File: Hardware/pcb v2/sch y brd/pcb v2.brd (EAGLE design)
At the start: 80 x 80 mm, 60 parts, among them J1 AVR_SPI_PRG_6PTH, J2 1981584-1, J3 HDMI, J4 HDMI, J5 JST-3, Q1 PMBT3904, Q2 PMBT3904, Q4 MC-306, U1 ATMEGA328P, U2 TXS0108EPWR-TSSOP20, U3 MB85RS16N, U4 ADP3338AKCZ-3.3RL7, U5 DS1307SO8, Y2 CSTCE16M0V53-R0 16MHZ

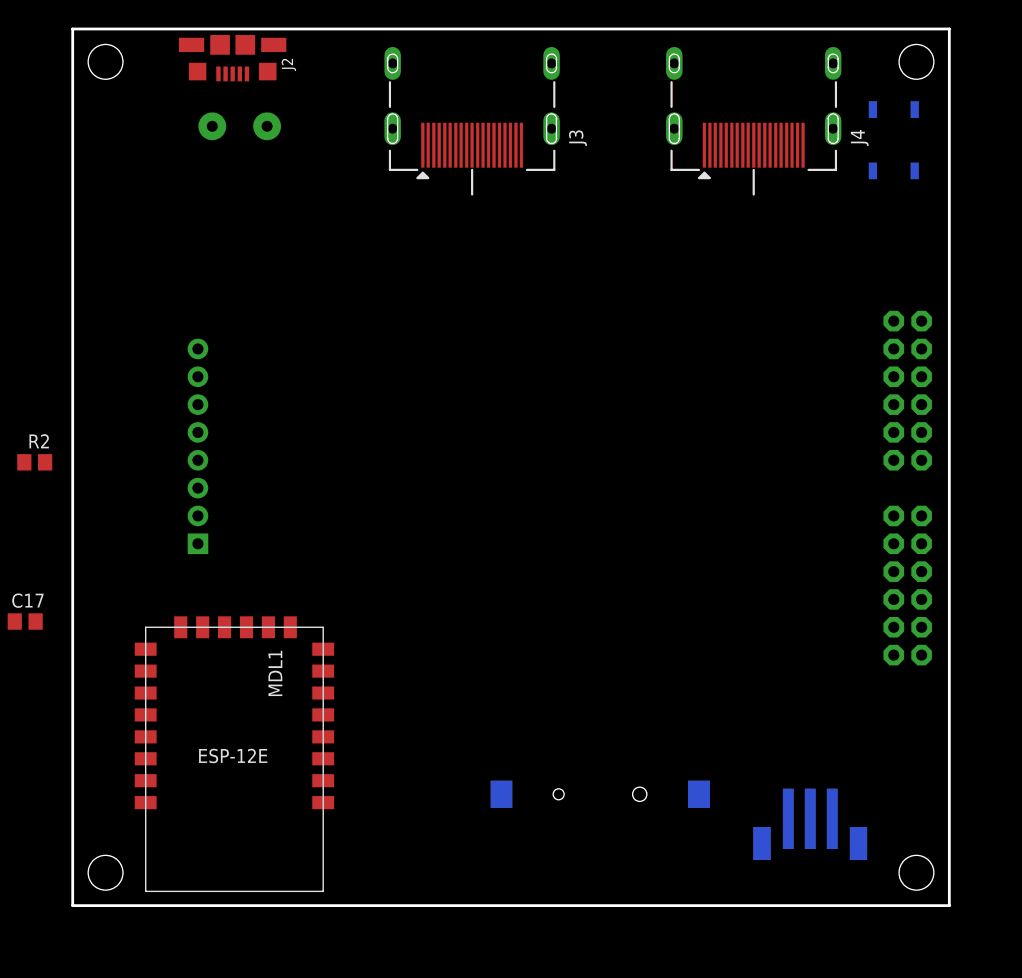
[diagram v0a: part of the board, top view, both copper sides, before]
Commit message: ruteo tdms
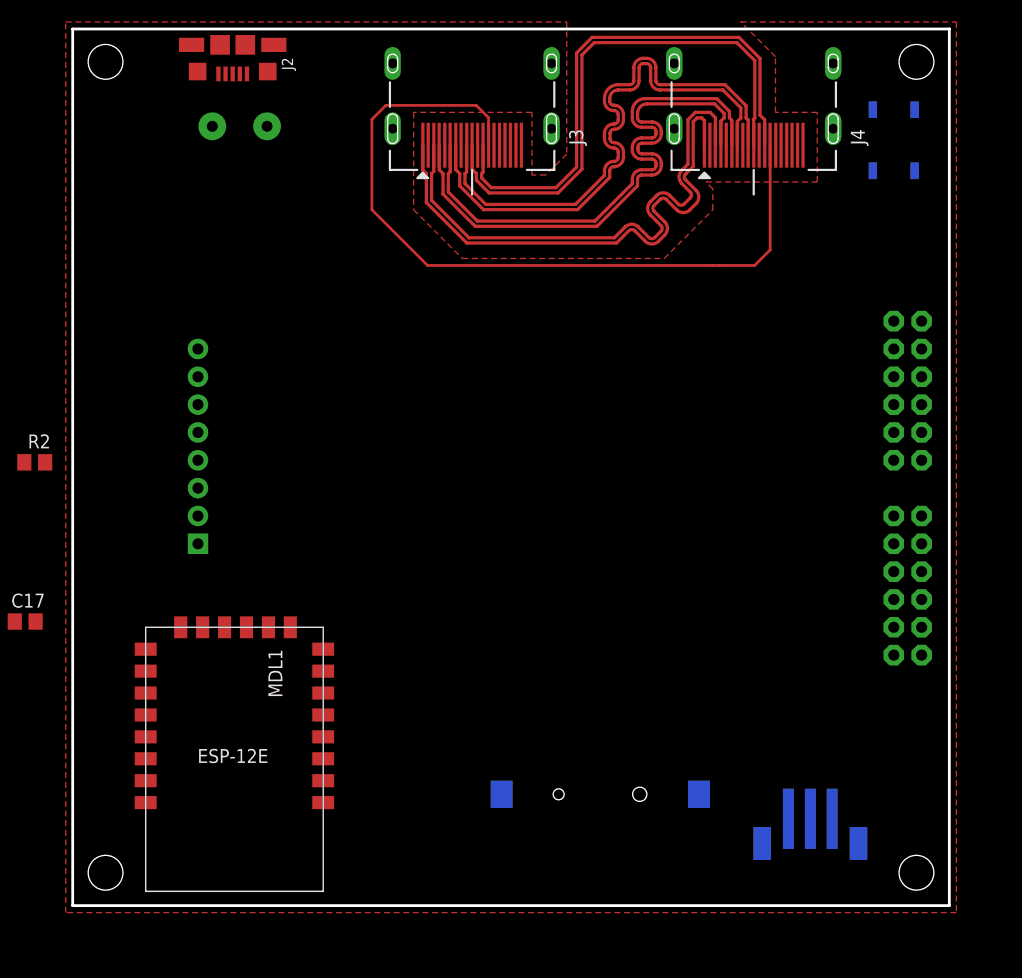
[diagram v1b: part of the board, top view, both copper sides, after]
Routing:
- net N$30: track 0.00 -> 71.0 mm
- net CLK_N: track 0.00 -> 49.5 mm
- net CLK_P: track 0.00 -> 49.5 mm
- net TX2_N: track 0.00 -> 49.2 mm
- net TX2_P: track 0.00 -> 49.2 mm
- net TX1_P: track 0.00 -> 49.1 mm
- net TX1_N: track 0.00 -> 49.1 mm
- net TX0_P: track 0.00 -> 48.9 mm
- net TX0_N: track 0.00 -> 48.7 mm
- added copper zone on layer 1, net GND
